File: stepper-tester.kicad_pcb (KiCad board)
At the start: 2 copper layers, 81.3 x 40.6 mm, 18 parts, among them J1 POWER, J2 Conn_01x04_Male, SW1 DIR SWITCH, SW2 ENABLE SWITCH, U1 NE555P, U2 AMS1117-5.0

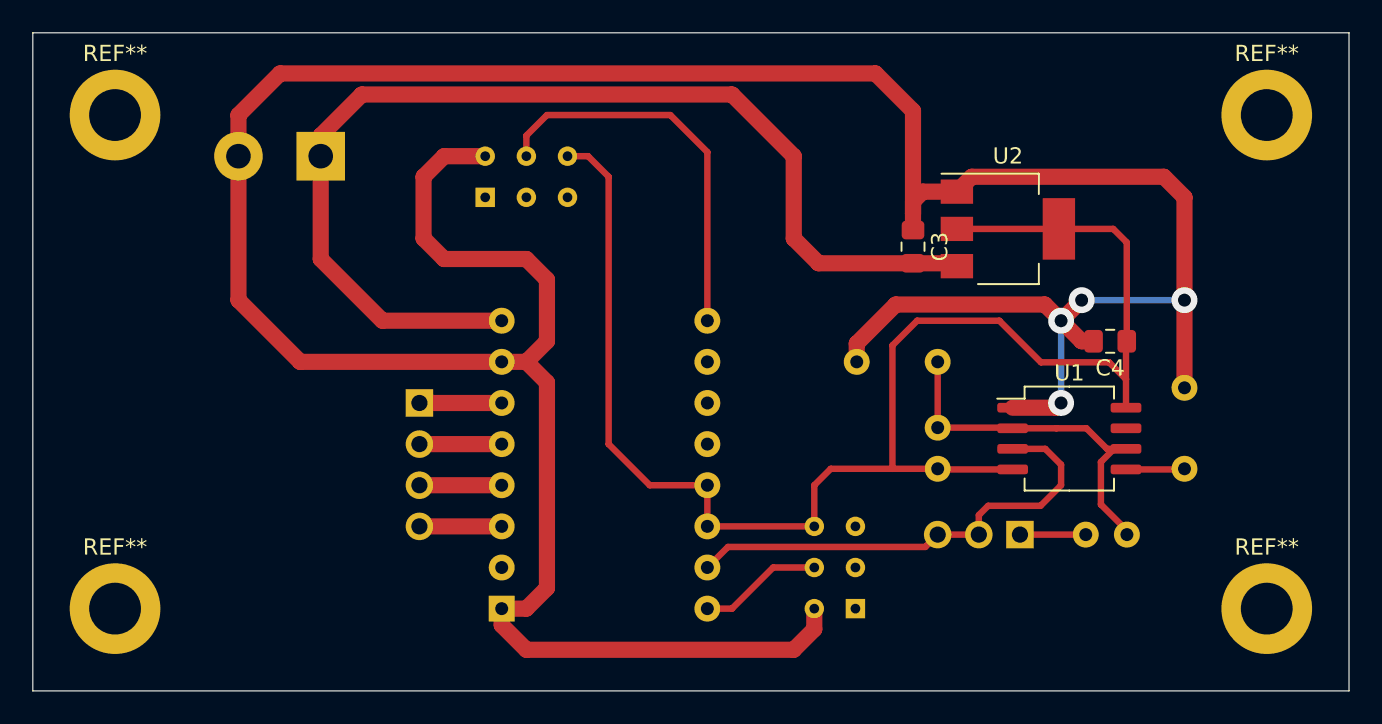
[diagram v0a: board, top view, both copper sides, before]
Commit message: PCB WIP
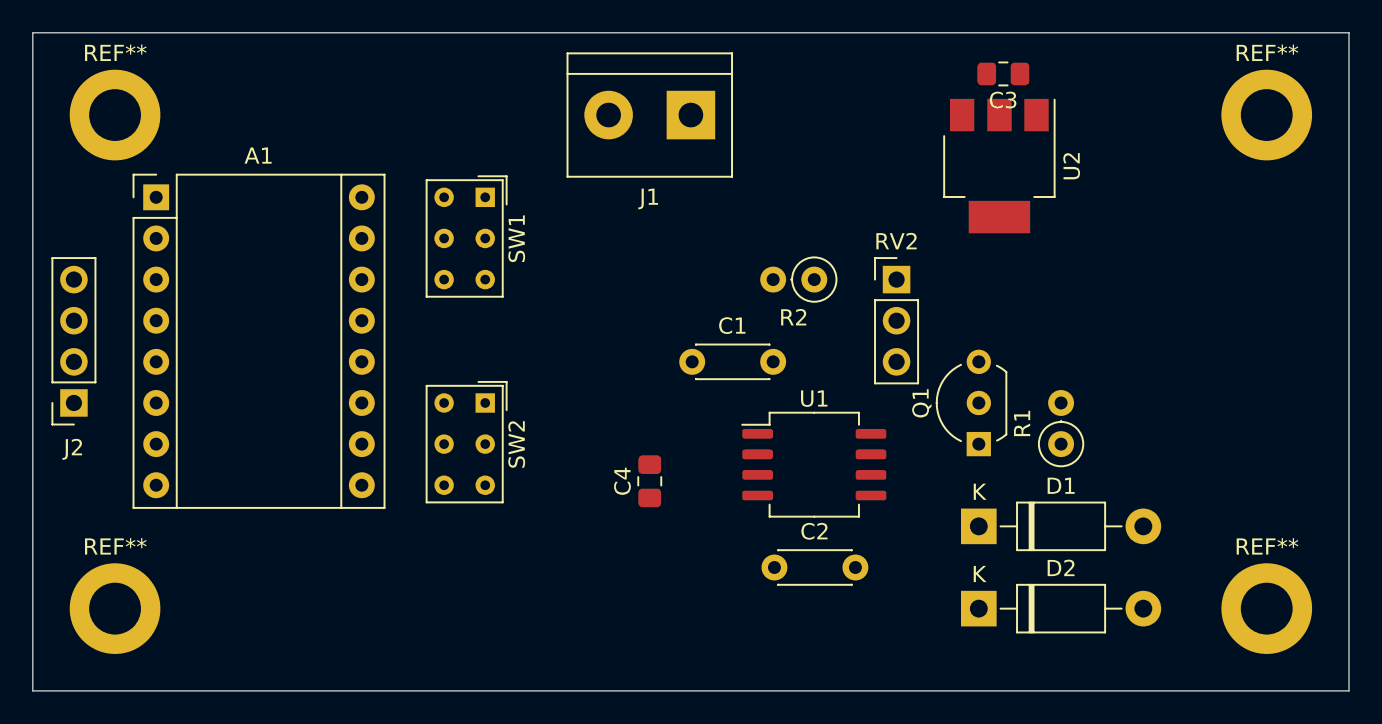
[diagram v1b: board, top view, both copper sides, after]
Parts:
- added D1: 1N5817, Diode_THT:D_DO-41_SOD81_P10.16mm_Horizontal, F.Cu at (127.0, 81.3)
- added D2: 1N5817, Diode_THT:D_DO-41_SOD81_P10.16mm_Horizontal, F.Cu at (127.0, 86.4)
- added Q1: BC547, Package_TO_SOT_THT:TO-92L_Inline_Wide, F.Cu at (127.0, 76.2)
- A1, C1, C2, J2, R2, RV2: moved to F.Cu
- J1: value POWER -> Barrel_Jack; moved to F.Cu
- R1: value 470K -> 1K; moved to F.Cu
- SW1: value DIR SWITCH -> SW_Push_DPDT; moved to F.Cu
- SW2: value ENABLE SWITCH -> SW_Push_DPDT; moved to F.Cu
- moved SW1 34.2 mm to (96.5, 61.0), turned to 270 degrees
- moved A1 33.2 mm to (76.2, 61.0)
- moved C4 29.7 mm to (106.7, 78.5), turned to 90 degrees
- moved C2 27.6 mm to (114.4, 83.8), turned to 0 degrees
- moved J1 23.0 mm to (109.2, 55.9)
- moved R2 23.0 mm to (116.8, 66.0), turned to 180 degrees
- moved J2 21.3 mm to (71.1, 73.7)
- moved RV2 17.5 mm to (121.9, 66.0), turned to 0 degrees
- moved U1 15.8 mm to (116.8, 77.5)
- moved SW2 12.7 mm to (96.5, 73.7), turned to 270 degrees
- moved C3 12.0 mm to (128.5, 53.3), turned to 180 degrees
- moved C1 10.2 mm to (109.3, 71.1)
- moved R1 7.69 mm to (132.1, 76.2), turned to 90 degrees
- moved U2 3.92 mm to (128.3, 59.0), turned to 270 degrees
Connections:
- R1 pad 1: Net-(C1-Pad2) -> 5V
- R1 pad 2: 5V -> Net-(D2-Pad2)
- RV2 pad 2: STEP -> Net-(D1-Pad2)
- RV2 pad 3: STEP -> Net-(D1-Pad2)
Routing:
- net GND: track 209.3 -> 0.00 mm, vias 4 -> 0
- net 5V: track 96.3 -> 0.00 mm
- net VMOT: track 68.1 -> 0.00 mm
- net STEP: track 29.3 -> 0.00 mm
- net EN: track 24.3 -> 0.00 mm
- net Net-(C1-Pad2): track 23.3 -> 0.00 mm
- net DIR: track 7.66 -> 0.00 mm
- net Net-(A1-Pad6): track 5.08 -> 0.00 mm
- net Net-(A1-Pad5): track 5.08 -> 0.00 mm
- net Net-(A1-Pad4): track 5.08 -> 0.00 mm
- net Net-(A1-Pad3): track 5.08 -> 0.00 mm
- net Net-(R2-Pad1): track 4.06 -> 0.00 mm
- net Net-(C2-Pad2): track 3.63 -> 0.00 mm
